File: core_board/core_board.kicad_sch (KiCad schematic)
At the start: 96 parts

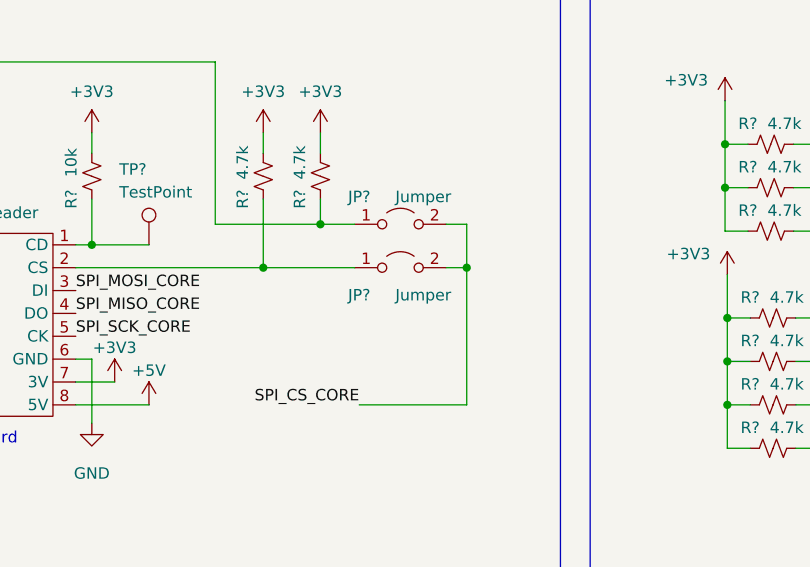
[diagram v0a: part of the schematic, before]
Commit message: last commit before starting layout
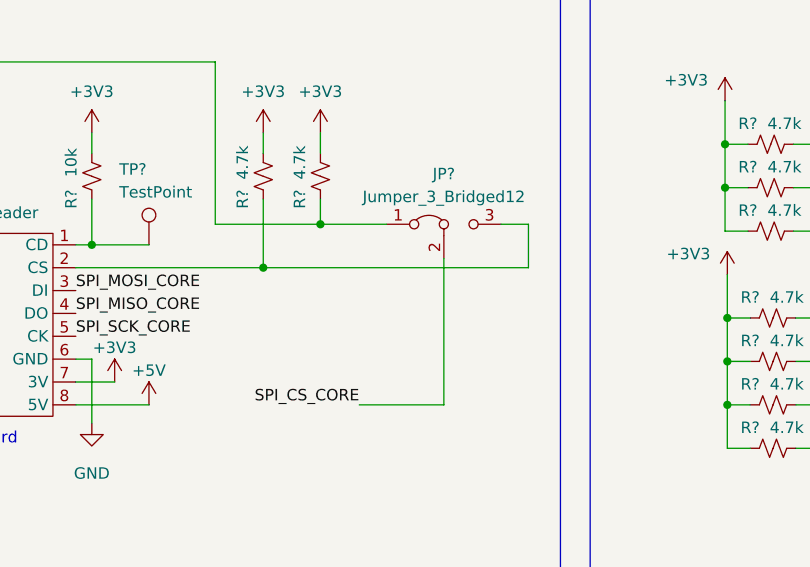
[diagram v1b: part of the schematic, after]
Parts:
- removed JP? (x2): Jumper, symbol Jumper:Jumper_2_Open
- added JP?: Jumper_3_Bridged12, symbol Jumper:Jumper_3_Bridged12
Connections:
- net SPI_CS_CORE: now also JP?.2 (C)
- net at R?.1, U?.2 (CS): now also JP?.3 (B)
- net at R?.1, U?.2 (CS): now also JP?.1 (A)
